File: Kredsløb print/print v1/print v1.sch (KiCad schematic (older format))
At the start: 70 parts, among them J1 Conn_01x01_Male, J2 Conn_01x01_Male, J3 Conn_01x01_Male, J4 Conn_01x01_Male, J5 Conn_01x01_Male, Q1 TIP127, Q2 TIP120, Q3 TIP120, Q4 TIP127, Q5 TIP120, U1 esp32, U2 4049

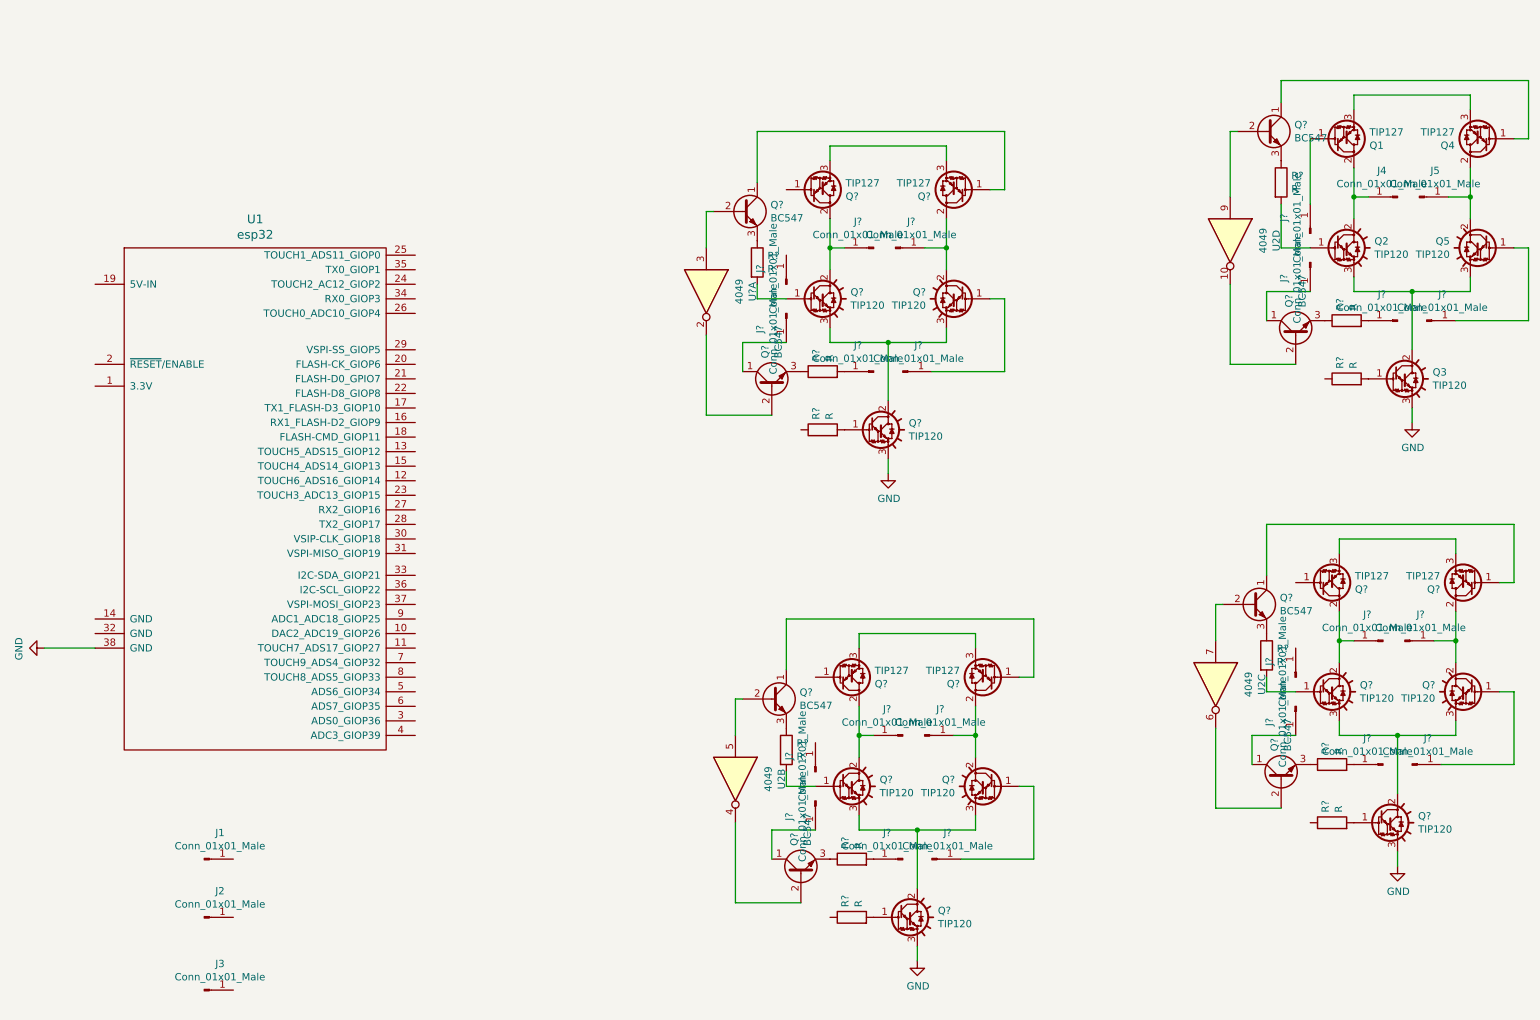
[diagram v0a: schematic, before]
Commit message: stuff
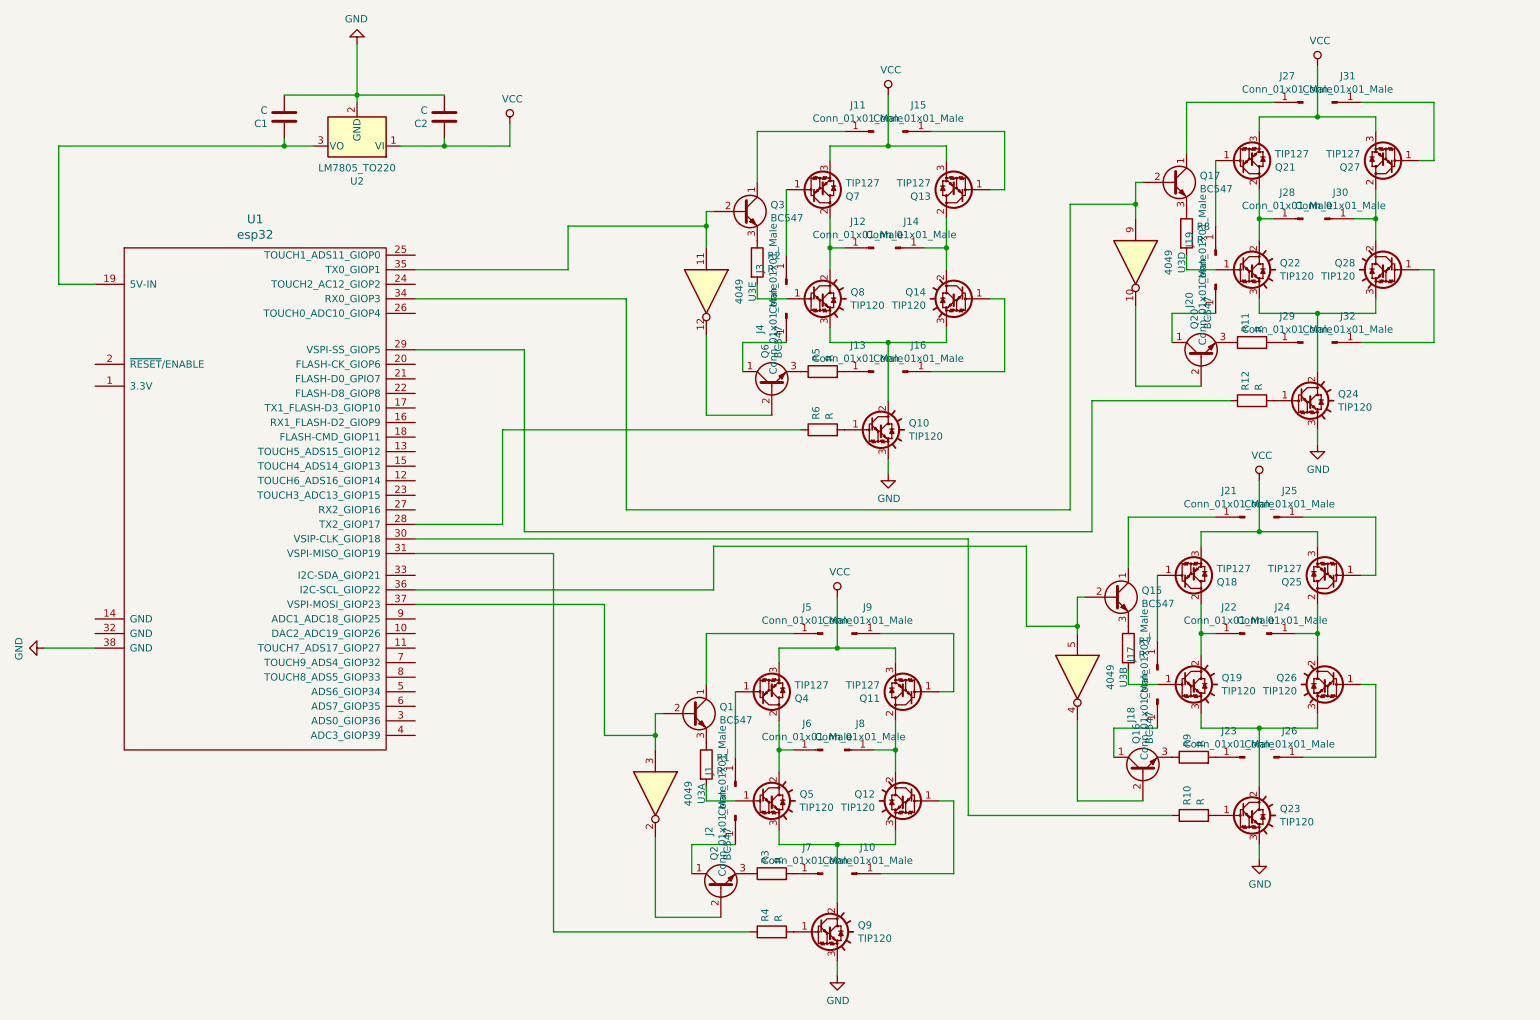
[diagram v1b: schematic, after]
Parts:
- removed J3, J4, J? (x16): Conn_01x01_Male, Connector_PinHeader_1.00mm:PinHeader_1x01_P1.00mm_Vertical, symbol Connector:Conn_01x01_Male
- removed Q1, Q? (x4): TIP127, Package_TO_SOT_THT:TO-220-3_Vertical, symbol 00-OTG-Transistor:TIP127
- removed Q2, Q3, Q? (x6): TIP120, TO_SOT_Packages_THT:TO-220_Vertical, symbol 00-OTG-Transistor:TIP120
- removed Q? (x6): BC547, Package_TO_SOT_THT:TO-92_Inline, symbol 00-OTG-Transistor:BC547
- removed R? (x9): R, symbol Device:R
- removed U2: 4049, Package_DIP:DIP-16_W7.62mm_LongPads, symbol 4xxx:4049
- added C1, C2: C, footprints otg:C_5.00mm, symbol Device:C
- added J10, J11, J15, J17, J18, J19, J20, J21, J22, J23, J24, J25, J26, J27, J28, J29, J30, J31, J32, J6, J7, J8, J9: Conn_01x01_Male, Connector_PinHeader_1.00mm:PinHeader_1x01_P1.00mm_Vertical, symbol Connector:Conn_01x01_Male
- added Q1, Q15, Q16, Q17, Q2, Q20: BC547, Package_TO_SOT_THT:TO-92_Inline, symbol 00-OTG-Transistor:BC547
- added Q11, Q18, Q21, Q25, Q27: TIP127, Package_TO_SOT_THT:TO-220-3_Vertical, symbol 00-OTG-Transistor:TIP127
- added Q12, Q19, Q22, Q23, Q24, Q26, Q28, Q9: TIP120, TO_SOT_Packages_THT:TO-220_Vertical, symbol 00-OTG-Transistor:TIP120
- added R1, R10, R11, R12, R3, R4, R7, R8, R9: R, symbol Device:R
- added U2: LM7805_TO220, Package_TO_SOT_THT:TO-220-3_Vertical, symbol Regulator_Linear:LM7805_TO220
- added unit 4 of U3
- added unit 2 of U3
- added unit 1 of U3
- gave numbers to parts that had none: 17
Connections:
- net GND: now also C1.2, C2.2, Q23.3 (E), Q24.3 (E), Q9.3 (E), U2.2 (GND)
- net at U1.19 (5V-IN): now also C1.1, U2.3 (VO)
- net at U1.28 (TX2_GIOP17): now also R6.1
- net at U1.29 (VSPI-SS_GIOP5): now also R12.1
- net at U1.30 (VSIP-CLK_GIOP18): now also R10.1
- net at U1.31 (VSPI-MISO_GIOP19): now also R4.1
- net at U1.34 (RX0_GIOP3): now also Q17.2 (B), U3.9
- net at U1.35 (TX0_GIOP1): now also Q3.2 (B), U3.11
- net at U1.36 (I2C-SCL_GIOP22): now also Q15.2 (B), U3.5
- net at U1.37 (VSPI-MOSI_GIOP23): now also Q1.2 (B), U3.3
- net at Q5.3 (E): now also Q12.3 (E), Q9.2 (C)
- net at Q5.1 (B): now also R1.2
- net at Q4.2 (C), Q5.2 (C): now also J6.1 (Pin_1); no longer J5.1 (Pin_1)
- net VCC: now reaches Q4.3 (E)
- net VCC: now also Q13.3 (E), Q7.3 (E), C2.1, Q11.3 (E), Q18.3 (E), Q21.3 (E), Q25.3 (E), Q27.3 (E), U2.1 (VI)
- net at Q4.1 (B): now also J1.1 (Pin_1)
- net at J2.1 (Pin_1): now also Q2.1 (C)
- net at Q13.1 (B): now also J15.1 (Pin_1); no longer Q3.1 (C)
- net at Q6.2 (B): now also U3.12; no longer U3.2
- net at J3.1 (Pin_1): now also Q7.1 (B)
- new net: J11.1 (Pin_1), Q3.1 (C)
- new net: Q22.1 (B), R8.2
- new net: J28.1 (Pin_1), Q21.2 (C), Q22.2 (C)
- new net: Q22.3 (E), Q24.2 (C), Q28.3 (E)
- new net: J32.1 (Pin_1), Q28.1 (B)
- new net: J30.1 (Pin_1), Q27.2 (C), Q28.2 (C)
- new net: Q24.1 (B), R12.2
- new net: Q20.2 (B), U3.10
- new net: J20.1 (Pin_1), Q20.1 (C)
- new net: Q20.3 (E), R11.1
- new net: J29.1 (Pin_1), R11.2
- new net: J27.1 (Pin_1), Q17.1 (C)
- new net: Q17.3 (E), R8.1
- new net: J19.1 (Pin_1), Q21.1 (B)
- new net: J31.1 (Pin_1), Q27.1 (B)
- new net: Q19.1 (B), R7.2
- new net: J22.1 (Pin_1), Q18.2 (C), Q19.2 (C)
- new net: Q19.3 (E), Q23.2 (C), Q26.3 (E)
- new net: J26.1 (Pin_1), Q26.1 (B)
- new net: J24.1 (Pin_1), Q25.2 (C), Q26.2 (C)
- new net: Q23.1 (B), R10.2
- new net: Q16.2 (B), U3.4
- new net: J18.1 (Pin_1), Q16.1 (C)
- new net: Q16.3 (E), R9.1
- new net: J23.1 (Pin_1), R9.2
- new net: J21.1 (Pin_1), Q15.1 (C)
- new net: Q15.3 (E), R7.1
- new net: J17.1 (Pin_1), Q18.1 (B)
- new net: J25.1 (Pin_1), Q25.1 (B)
- new net: J10.1 (Pin_1), Q12.1 (B)
- new net: J8.1 (Pin_1), Q11.2 (C), Q12.2 (C)
- new net: Q9.1 (B), R4.2
- new net: Q2.2 (B), U3.2
- new net: Q2.3 (E), R3.1
- new net: J7.1 (Pin_1), R3.2
- new net: J5.1 (Pin_1), Q1.1 (C)
- new net: Q1.3 (E), R1.1
- new net: J9.1 (Pin_1), Q11.1 (B)

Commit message: kredsløb og ny motor mount
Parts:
- C1, C2: footprint footprints otg:C_5.00mm -> Custom footprints:C_6.00mm
- Q10, Q12, Q14, Q19, Q22, Q23, Q24, Q26, Q28, Q5, Q8, Q9: footprint TO_SOT_Packages_THT:TO-220_Vertical -> Package_TO_SOT_THT:TO-220-3_Vertical
- R1, R10, R11, R12, R2, R3, R4, R5, R6, R7, R8, R9: footprint (none) -> footprints otg:R_vandret
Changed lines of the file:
@@
 F 0 "Q8" H 6241 2446 50  0000 L CNN
 F 1 "TIP120" H 6241 2355 50  0000 L CNN
-F 2 "TO_SOT_Packages_THT:TO-220_Vertical" H 6250 2325 50  0001 L CIN
+F 2 "Package_TO_SOT_THT:TO-220-3_Vertical" H 6250 2325 50  0001 L CIN
 F 3 "http://www.fairchildsemi.com/ds/TI/TIP120.pdf" H 6000 2400 50  0001 L CNN
 	1    6000 2400
@@
 F 0 "Q14" H 7241 2446 50  0000 L CNN
 F 1 "TIP120" H 7241 2355 50  0000 L CNN
-F 2 "TO_SOT_Packages_THT:TO-220_Vertical" H 7250 2325 50  0001 L CIN
+F 2 "Package_TO_SOT_THT:TO-220-3_Vertical" H 7250 2325 50  0001 L CIN
 F 3 "http://www.fairchildsemi.com/ds/TI/TIP120.pdf" H 7000 2400 50  0001 L CNN
 	1    7000 2400
@@
 F 0 "Q10" H 6641 3346 50  0000 L CNN
 F 1 "TIP120" H 6641 3255 50  0000 L CNN
-F 2 "TO_SOT_Packages_THT:TO-220_Vertical" H 6650 3225 50  0001 L CIN
+F 2 "Package_TO_SOT_THT:TO-220-3_Vertical" H 6650 3225 50  0001 L CIN
 F 3 "http://www.fairchildsemi.com/ds/TI/TIP120.pdf" H 6400 3300 50  0001 L CNN
 	1    6400 3300
@@
 F 0 "R5" H 6120 2946 50  0000 L CNN
 F 1 "R" H 6120 2855 50  0000 L CNN
-F 2 "" V 5980 2900 50  0001 C CNN
+F 2 "footprints otg:R_vandret" V 5980 2900 50  0001 C CNN
 F 3 "~" H 6050 2900 50  0001 C CNN
 	1    6050 2900
@@
 F 0 "R2" H 5670 2196 50  0000 L CNN
 F 1 "R" H 5670 2105 50  0000 L CNN
-F 2 "" V 5530 2150 50  0001 C CNN
+F 2 "footprints otg:R_vandret" V 5530 2150 50  0001 C CNN
 F 3 "~" H 5600 2150 50  0001 C CNN
 	1    5600 2150
@@
 F 0 "R6" H 6120 3346 50  0000 L CNN
 F 1 "R" H 6120 3255 50  0000 L CNN
-F 2 "" V 5980 3300 50  0001 C CNN
+F 2 "footprints otg:R_vandret" V 5980 3300 50  0001 C CNN
 F 3 "~" H 6050 3300 50  0001 C CNN
 	1    6050 3300
@@
 F 0 "C2" H 3565 1196 50  0000 L CNN
 F 1 "C" H 3565 1105 50  0000 L CNN
-F 2 "footprints otg:C_5.00mm" H 3488 1000 50  0001 C CNN
+F 2 "Custom footprints:C_6.00mm" H 3488 1000 50  0001 C CNN
 F 3 "~" H 3450 1150 50  0001 C CNN
 	1    3450 1150
@@
 F 0 "C1" H 2465 1196 50  0000 L CNN
 F 1 "C" H 2465 1105 50  0000 L CNN
-F 2 "footprints otg:C_5.00mm" H 2388 1000 50  0001 C CNN
+F 2 "Custom footprints:C_6.00mm" H 2388 1000 50  0001 C CNN
 F 3 "~" H 2350 1150 50  0001 C CNN
 	1    2350 1150
@@
 F 0 "Q22" H 9191 2246 50  0000 L CNN
 F 1 "TIP120" H 9191 2155 50  0000 L CNN
-F 2 "TO_SOT_Packages_THT:TO-220_Vertical" H 9200 2125 50  0001 L CIN
+F 2 "Package_TO_SOT_THT:TO-220-3_Vertical" H 9200 2125 50  0001 L CIN
 F 3 "http://www.fairchildsemi.com/ds/TI/TIP120.pdf" H 8950 2200 50  0001 L CNN
 	1    8950 2200
@@
 F 0 "Q28" H 10191 2246 50  0000 L CNN
 F 1 "TIP120" H 10191 2155 50  0000 L CNN
-F 2 "TO_SOT_Packages_THT:TO-220_Vertical" H 10200 2125 50  0001 L CIN
+F 2 "Package_TO_SOT_THT:TO-220-3_Vertical" H 10200 2125 50  0001 L CIN
 F 3 "http://www.fairchildsemi.com/ds/TI/TIP120.pdf" H 9950 2200 50  0001 L CNN
 	1    9950 2200
@@
 F 0 "Q24" H 9591 3146 50  0000 L CNN
 F 1 "TIP120" H 9591 3055 50  0000 L CNN
-F 2 "TO_SOT_Packages_THT:TO-220_Vertical" H 9600 3025 50  0001 L CIN
+F 2 "Package_TO_SOT_THT:TO-220-3_Vertical" H 9600 3025 50  0001 L CIN
 F 3 "http://www.fairchildsemi.com/ds/TI/TIP120.pdf" H 9350 3100 50  0001 L CNN
 	1    9350 3100
@@
 F 0 "R11" H 9070 2746 50  0000 L CNN
 F 1 "R" H 9070 2655 50  0000 L CNN
-F 2 "" V 8930 2700 50  0001 C CNN
+F 2 "footprints otg:R_vandret" V 8930 2700 50  0001 C CNN
 F 3 "~" H 9000 2700 50  0001 C CNN
 	1    9000 2700
@@
 F 0 "R8" H 8620 1996 50  0000 L CNN
 F 1 "R" H 8620 1905 50  0000 L CNN
-F 2 "" V 8480 1950 50  0001 C CNN
+F 2 "footprints otg:R_vandret" V 8480 1950 50  0001 C CNN
 F 3 "~" H 8550 1950 50  0001 C CNN
 	1    8550 1950
@@
 F 0 "R12" H 9070 3146 50  0000 L CNN
 F 1 "R" H 9070 3055 50  0000 L CNN
-F 2 "" V 8930 3100 50  0001 C CNN
+F 2 "footprints otg:R_vandret" V 8930 3100 50  0001 C CNN
 F 3 "~" H 9000 3100 50  0001 C CNN
 	1    9000 3100
@@
 F 0 "Q19" H 8791 5096 50  0000 L CNN
 F 1 "TIP120" H 8791 5005 50  0000 L CNN
-F 2 "TO_SOT_Packages_THT:TO-220_Vertical" H 8800 4975 50  0001 L CIN
+F 2 "Package_TO_SOT_THT:TO-220-3_Vertical" H 8800 4975 50  0001 L CIN
 F 3 "http://www.fairchildsemi.com/ds/TI/TIP120.pdf" H 8550 5050 50  0001 L CNN
 	1    8550 5050
@@
 F 0 "Q26" H 9791 5096 50  0000 L CNN
 F 1 "TIP120" H 9791 5005 50  0000 L CNN
-F 2 "TO_SOT_Packages_THT:TO-220_Vertical" H 9800 4975 50  0001 L CIN
+F 2 "Package_TO_SOT_THT:TO-220-3_Vertical" H 9800 4975 50  0001 L CIN
 F 3 "http://www.fairchildsemi.com/ds/TI/TIP120.pdf" H 9550 5050 50  0001 L CNN
 	1    9550 5050
@@
 F 0 "Q23" H 9191 5996 50  0000 L CNN
 F 1 "TIP120" H 9191 5905 50  0000 L CNN
-F 2 "TO_SOT_Packages_THT:TO-220_Vertical" H 9200 5875 50  0001 L CIN
+F 2 "Package_TO_SOT_THT:TO-220-3_Vertical" H 9200 5875 50  0001 L CIN
 F 3 "http://www.fairchildsemi.com/ds/TI/TIP120.pdf" H 8950 5950 50  0001 L CNN
 	1    8950 5950
@@
 F 0 "R9" H 8670 5596 50  0000 L CNN
 F 1 "R" H 8670 5505 50  0000 L CNN
-F 2 "" V 8530 5550 50  0001 C CNN
+F 2 "footprints otg:R_vandret" V 8530 5550 50  0001 C CNN
 F 3 "~" H 8600 5550 50  0001 C CNN
 	1    8600 5550
@@
 F 0 "R7" H 8220 4846 50  0000 L CNN
 F 1 "R" H 8220 4755 50  0000 L CNN
-F 2 "" V 8080 4800 50  0001 C CNN
+F 2 "footprints otg:R_vandret" V 8080 4800 50  0001 C CNN
 F 3 "~" H 8150 4800 50  0001 C CNN
 	1    8150 4800
@@
 F 0 "R10" H 8670 5996 50  0000 L CNN
 F 1 "R" H 8670 5905 50  0000 L CNN
-F 2 "" V 8530 5950 50  0001 C CNN
+F 2 "footprints otg:R_vandret" V 8530 5950 50  0001 C CNN
 F 3 "~" H 8600 5950 50  0001 C CNN
 	1    8600 5950
@@
 F 0 "Q5" H 5891 5896 50  0000 L CNN
 F 1 "TIP120" H 5891 5805 50  0000 L CNN
-F 2 "TO_SOT_Packages_THT:TO-220_Vertical" H 5900 5775 50  0001 L CIN
+F 2 "Package_TO_SOT_THT:TO-220-3_Vertical" H 5900 5775 50  0001 L CIN
 F 3 "http://www.fairchildsemi.com/ds/TI/TIP120.pdf" H 5650 5850 50  0001 L CNN
 	1    5650 5850
@@
 F 0 "Q12" H 6891 5896 50  0000 L CNN
 F 1 "TIP120" H 6891 5805 50  0000 L CNN
-F 2 "TO_SOT_Packages_THT:TO-220_Vertical" H 6900 5775 50  0001 L CIN
+F 2 "Package_TO_SOT_THT:TO-220-3_Vertical" H 6900 5775 50  0001 L CIN
 F 3 "http://www.fairchildsemi.com/ds/TI/TIP120.pdf" H 6650 5850 50  0001 L CNN
 	1    6650 5850
@@
 F 0 "Q9" H 6291 6796 50  0000 L CNN
 F 1 "TIP120" H 6291 6705 50  0000 L CNN
-F 2 "TO_SOT_Packages_THT:TO-220_Vertical" H 6300 6675 50  0001 L CIN
+F 2 "Package_TO_SOT_THT:TO-220-3_Vertical" H 6300 6675 50  0001 L CIN
 F 3 "http://www.fairchildsemi.com/ds/TI/TIP120.pdf" H 6050 6750 50  0001 L CNN
 	1    6050 6750
@@
 F 0 "R3" H 5770 6396 50  0000 L CNN
 F 1 "R" H 5770 6305 50  0000 L CNN
-F 2 "" V 5630 6350 50  0001 C CNN
+F 2 "footprints otg:R_vandret" V 5630 6350 50  0001 C CNN
 F 3 "~" H 5700 6350 50  0001 C CNN
 	1    5700 6350
@@
 F 0 "R1" H 5320 5646 50  0000 L CNN
 F 1 "R" H 5320 5555 50  0000 L CNN
-F 2 "" V 5180 5600 50  0001 C CNN
+F 2 "footprints otg:R_vandret" V 5180 5600 50  0001 C CNN
 F 3 "~" H 5250 5600 50  0001 C CNN
 	1    5250 5600
@@
 F 0 "R4" H 5770 6796 50  0000 L CNN
 F 1 "R" H 5770 6705 50  0000 L CNN
-F 2 "" V 5630 6750 50  0001 C CNN
+F 2 "footprints otg:R_vandret" V 5630 6750 50  0001 C CNN
 F 3 "~" H 5700 6750 50  0001 C CNN
 	1    5700 6750
